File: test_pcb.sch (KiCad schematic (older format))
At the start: 24 parts, among them J1 Conn_01x04_Male, J11 Conn_01x20_Female, J8 Conn_01x20_Female, SW1 on/off, SW2 on/off

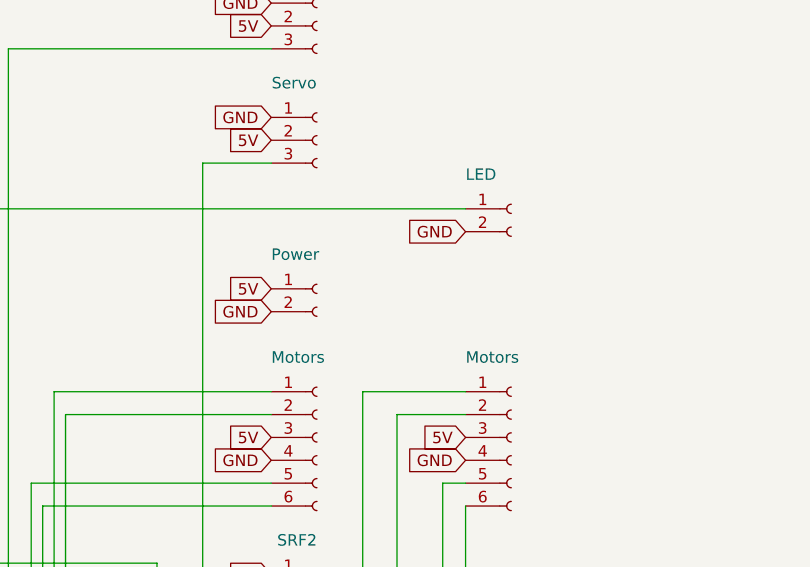
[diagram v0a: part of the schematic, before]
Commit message: small text changes
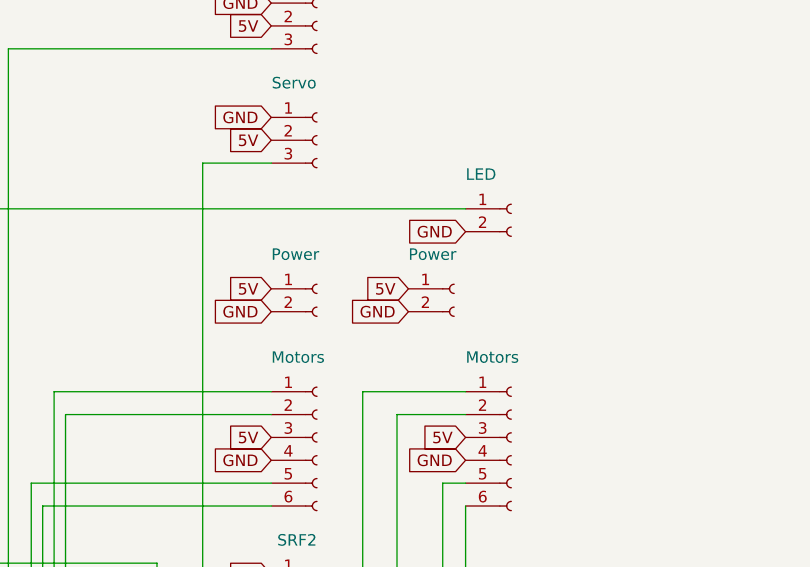
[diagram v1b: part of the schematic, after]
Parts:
- added Power?: Power, Connector_PinSocket_2.54mm:PinSocket_1x02_P2.54mm_Vertical, symbol Connector:Conn_01x02_Female
- gave numbers to parts that had none: 1
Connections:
- net 5V: now also Power?.1 (Pin_1)
- net GND: now also Power?.2 (Pin_2)
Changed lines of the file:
@@
 Connection ~ 3900 4100
 $Comp
-L Connector:Conn_01x02_Female Power?
+L Connector:Conn_01x02_Female Power2
 U 1 1 601D6728
 P 6500 2050
-F 0 "Power?" H 6528 2026 50  0001 L CNN
+F 0 "Power2" H 6528 2026 50  0001 L CNN
 F 1 "LED" H 6300 2200 50  0000 L CNN
 F 2 "Connector_PinHeader_2.54mm:PinHeader_1x02_P2.54mm_Vertical" H 6500 2050 50  0001 C CNN
@@
 Wire Wire Line
 	3150 2050 6300 2050
+$Comp
+L Connector:Conn_01x02_Female Power?
+U 1 1 6021D8FD
+P 6250 2400
+F 0 "Power?" H 6278 2376 50  0001 L CNN
+F 1 "Power" H 6050 2550 50  0000 L CNN
+F 2 "Connector_PinSocket_2.54mm:PinSocket_1x02_P2.54mm_Vertical" H 6250 2400 50  0001 C CNN
+F 3 "~" H 6250 2400 50  0001 C CNN
+	1    6250 2400
+	1    0    0    -1
+$EndComp
+Text GLabel 6050 2400 0    50   Input ~ 0
+5V
+Text GLabel 6050 2500 0    50   Input ~ 0
+GND
 $EndSCHEMATC
